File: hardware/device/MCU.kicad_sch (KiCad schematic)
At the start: 25 parts, among them SW24 NRST, U1 BMDU, U18 STM32H743ZIT6

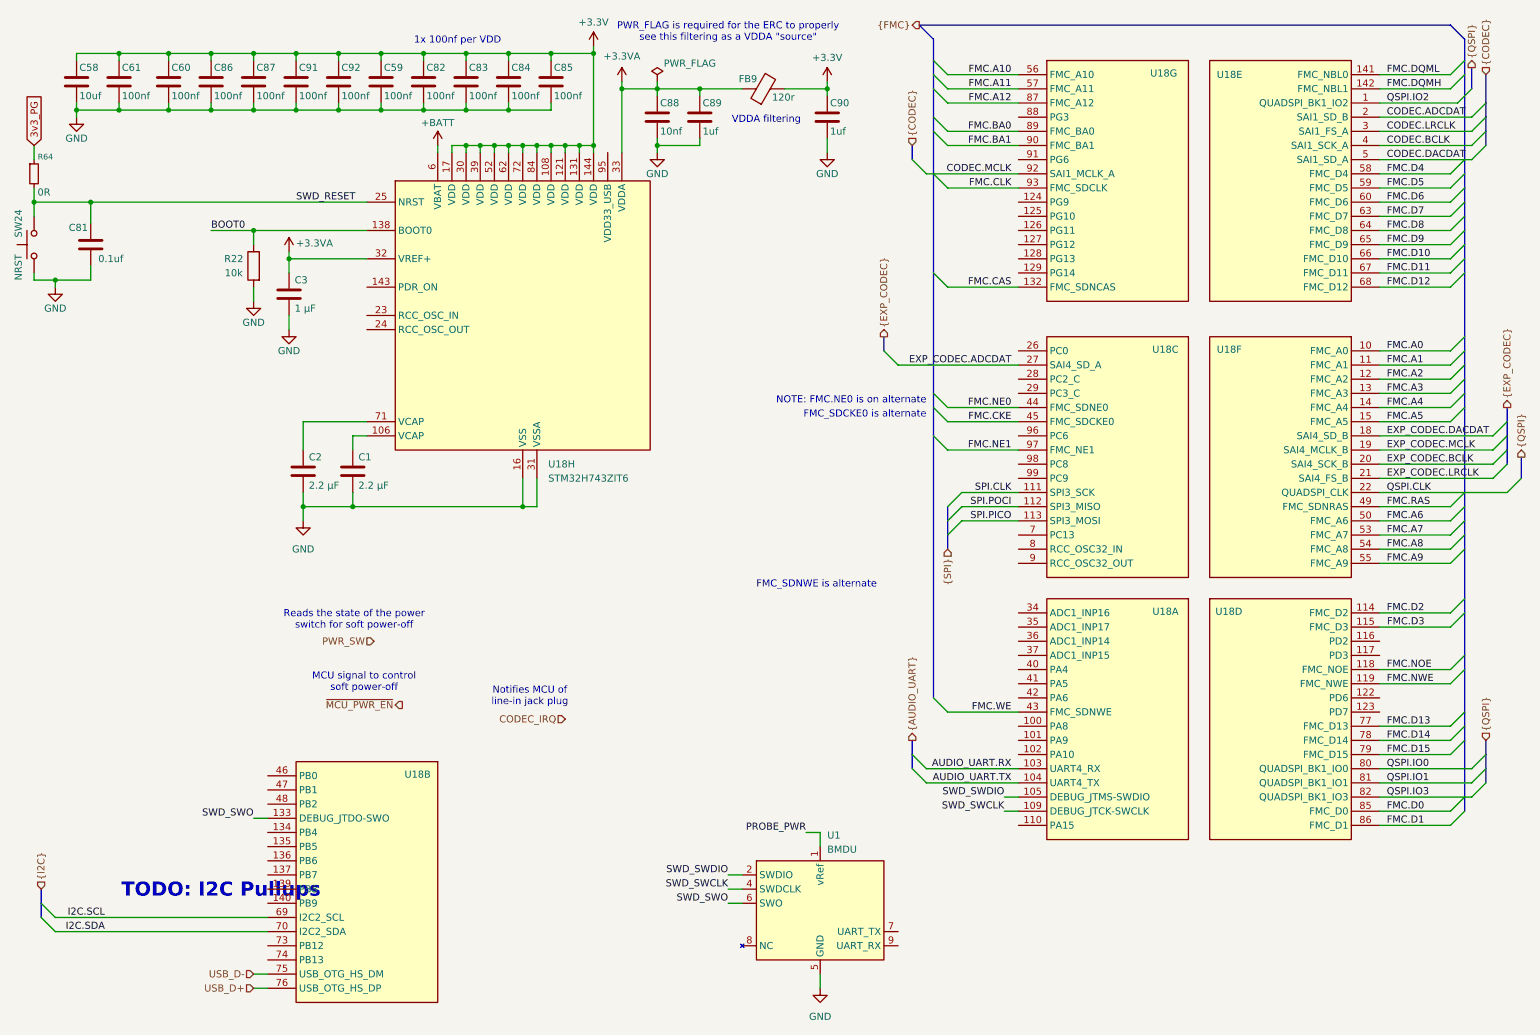
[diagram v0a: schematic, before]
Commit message: feat: add ESD filter
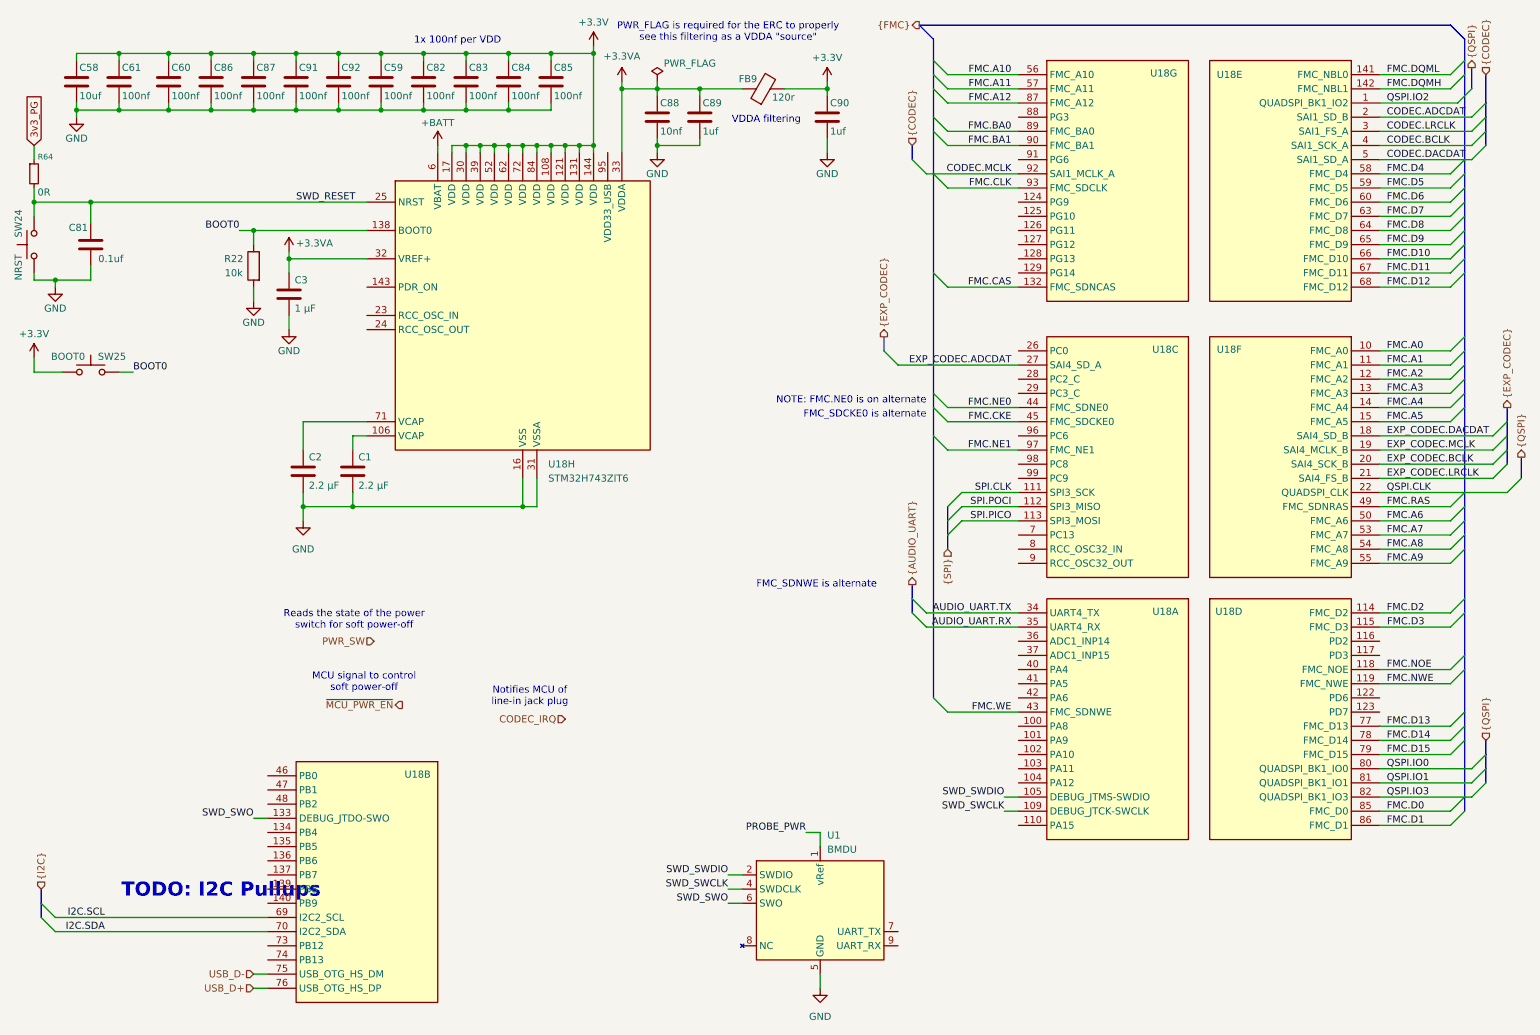
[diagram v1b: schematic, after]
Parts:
- added SW25: BOOT0, Button_Switch_SMD:SW_SPST_B3U-1000P, symbol Switch:SW_Push
- SW24: footprint (none) -> Button_Switch_SMD:SW_SPST_B3U-1000P
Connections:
- net +3.3V: now also SW25.1
- net AUDIO_UART.RX: now also U18.35 (PA1); no longer U18.103 (PA11)
- net AUDIO_UART.TX: now also U18.34 (PA0); no longer U18.104 (PA12)
- net BOOT0: now also SW25.2
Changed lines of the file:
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@@
 	)
 	(bus_entry
-		(at 176.53 147.32)
+		(at 176.53 121.92)
 		(size 2.54 2.54)
 		(stroke
@@
 	)
 	(bus_entry
-		(at 179.07 152.4)
+		(at 179.07 121.92)
 		(size -2.54 -2.54)
 		(stroke
@@
 	(bus
 		(pts
-			(xy 176.53 147.32) (xy 176.53 149.86)
-		)
-		(stroke
-			(width 0)
-			(type default)
-		)
-	)
-	(bus
-		(pts
-			(xy 176.53 144.78) (xy 176.53 147.32)
+			(xy 176.53 119.38) (xy 176.53 121.92)
 		)
 		(stroke
@@
 	(wire
 		(pts
+			(xy 24.13 78.74) (xy 19.05 78.74)
+		)
+		(stroke
+			(width 0)
+			(type default)
+		)
+	)
+	(wire
+		(pts
 			(xy 161.29 36.83) (xy 161.29 39.37)
 		)
@@
 		)
 	)
+	(bus
+		(pts
+			(xy 176.53 116.84) (xy 176.53 119.38)
+		)
+		(stroke
+			(width 0)
+			(type default)
+		)
+	)
 	(wire
 		(pts
@@
 	(wire
 		(pts
+			(xy 34.29 78.74) (xy 36.83 78.74)
+		)
+		(stroke
+			(width 0)
+			(type default)
+		)
+	)
+	(wire
+		(pts
 			(xy 138.43 36.83) (xy 138.43 38.1)
 		)
@@
 	(wire
 		(pts
-			(xy 179.07 152.4) (xy 195.58 152.4)
+			(xy 179.07 121.92) (xy 195.58 121.92)
 		)
 		(stroke
@@
 	(wire
 		(pts
-			(xy 50.8 53.34) (xy 58.42 53.34)
+			(xy 55.88 53.34) (xy 58.42 53.34)
 		)
 		(stroke
@@
 	(wire
 		(pts
-			(xy 179.07 149.86) (xy 195.58 149.86)
+			(xy 179.07 124.46) (xy 195.58 124.46)
 		)
 		(stroke
@@
 		)
 	)
+	(wire
+		(pts
+			(xy 19.05 76.2) (xy 19.05 78.74)
+		)
+		(stroke
+			(width 0)
+			(type default)
+		)
+	)
 	(bus
 		(pts
@@
 	)
 	(label "AUDIO_UART.RX"
-		(at 194.31 149.86 180)
+		(at 194.31 124.46 180)
 		(effects
 			(font
@@
 	)
 	(label "AUDIO_UART.TX"
-		(at 194.31 152.4 180)
+		(at 194.31 121.92 180)
 		(effects
 			(font
@@
 		)
 	)
+	(label "BOOT0"
+		(at 36.83 78.74 0)
+		(effects
+			(font
+				(size 1.27 1.27)
+			)
+			(justify left bottom)
+		)
+	)
 	(label "EXP_CODEC.LRCLK"
 		(at 261.62 97.79 0)
@@
 	)
 	(label "BOOT0"
-		(at 50.8 53.34 0)
+		(at 55.88 53.34 180)
 		(effects
 			(font
 				(size 1.27 1.27)
 			)
-			(justify left bottom)
+			(justify right bottom)
 		)
 	)
@@
 	(hierarchical_label "{AUDIO_UART}"
 		(shape output)
-		(at 176.53 144.78 90)
+		(at 176.53 116.84 90)
 		(effects
 			(font
@@
 	)
 	(symbol
+		(lib_id "power:+3.3V")
+		(at 19.05 76.2 0)
+		(unit 1)
+		(exclude_from_sim no)
+		(in_bom yes)
+		(on_board yes)
+		(dnp no)
+		(property "Reference" "#PWR0126"
+			(at 19.05 80.01 0)
+			(effects
+				(font
+					(size 1.27 1.27)
+				)
+				(hide yes)
+			)
+		)
+		(property "Value" "+3.3V"
+			(at 19.05 71.882 0)
+			(effects
+				(font
+					(size 1.27 1.27)
+				)
+			)
+		)
+		(property "Footprint" ""
+			(at 19.05 76.2 0)
+			(effects
+				(font
+					(size 1.27 1.27)
+				)
+				(hide yes)
+			)
+		)
+		(property "Datasheet" ""
+			(at 19.05 76.2 0)
+			(effects
+				(font
+					(size 1.27 1.27)
+				)
+				(hide yes)
+			)
+		)
+		(property "Description" "Power symbol creates a global label with name \"+3.3V\""
+			(at 19.05 76.2 0)
+			(effects
+				(font
+					(size 1.27 1.27)
+				)
+				(hide yes)
+			)
+		)
+		(pin "1"
+		)
+		(instances
+			(project "pocket_synth"
+				(path "/485383b8-00f4-4405-b270-de249939cff4/0f59ca20-5500-4399-8ffa-55aebf6eb4ee"
+					(reference "#PWR0126")
+					(unit 1)
+				)
+			)
+		)
+	)
+	(symbol
 		(lib_id "Switch:SW_Push")
 		(at 19.05 55.88 90)
@@
 			)
 		)
-		(property "Footprint" ""
+		(property "Footprint" "Button_Switch_SMD:SW_SPST_B3U-1000P"
 			(at 13.97 55.88 0)
 			(effects
@@
 	)
 	(symbol
+		(lib_id "Switch:SW_Push")
+		(at 29.21 78.74 0)
+		(unit 1)
+		(exclude_from_sim no)
+		(in_bom yes)
+		(on_board yes)
+		(dnp no)
+		(property "Reference" "SW25"
+			(at 33.02 75.946 0)
+			(effects
+				(font
+					(size 1.27 1.27)
+				)
+			)
+		)
+		(property "Value" "BOOT0"
+			(at 25.146 75.946 0)
+			(effects
+				(font
+					(size 1.27 1.27)
+				)
+			)
+		)
+		(property "Footprint" "Button_Switch_SMD:SW_SPST_B3U-1000P"
+			(at 29.21 73.66 0)
+			(effects
+				(font
+					(size 1.27 1.27)
+				)
+				(hide yes)
+			)
+		)
+		(property "Datasheet" "~"
+			(at 29.21 73.66 0)
+			(effects
+				(font
+					(size 1.27 1.27)
+				)
+				(hide yes)
+			)
+		)
+		(property "Description" "Push button switch, generic, two pins"
+			(at 29.21 78.74 0)
+			(effects
+				(font
+					(size 1.27 1.27)
+				)
+				(hide yes)
+			)
+		)
+		(property "Height" ""
+			(at 29.21 78.74 0)
+			(effects
+				(font
+					(size 1.27 1.27)
+				)
+			)
+		)
+		(property "Manufacturer_Name" ""
+			(at 29.21 78.74 0)
+			(effects
+				(font
+					(size 1.27 1.27)
+				)
+			)
+		)
+		(property "Manufacturer_Part_Number" ""
+			(at 29.21 78.74 0)
+			(effects
+				(font
+					(size 1.27 1.27)
+				)
+			)
+		)
+		(property "Mouser Part Number" ""
+			(at 29.21 78.74 0)
+			(effects
+				(font
+					(size 1.27 1.27)
+				)
+			)
+		)
+		(property "Mouser Price/Stock" ""
+			(at 29.21 78.74 0)
+			(effects
+				(font
+					(size 1.27 1.27)
+				)
+			)
+		)
+		(pin "2"
+		)
+		(pin "1"
+		)
+		(instances
+			(project "pocket_synth"
+				(path "/485383b8-00f4-4405-b270-de249939cff4/0f59ca20-5500-4399-8ffa-55aebf6eb4ee"
+					(reference "SW25")
+					(unit 1)
+				)
+			)
+		)
+	)
+	(symbol
 		(lib_id "power:+3.3V")
 		(at 161.29 26.67 0)
@@
 		)
 		(pin "34"
-			(alternate "ADC1_INP16")
+			(alternate "UART4_TX")
 		)
 		(pin "35"
-			(alternate "ADC1_INP17")
+			(alternate "UART4_RX")
 		)
 		(pin "36"
@@
 		)
 		(pin "103"
-			(alternate "UART4_RX")
+			(alternate "PA11")
 		)
 		(pin "104"
-			(alternate "UART4_TX")
+			(alternate "PA12")
 		)
 		(pin "105"
